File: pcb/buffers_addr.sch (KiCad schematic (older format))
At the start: 24 parts, among them U3 74LVCH162245A, U4 74LVCH162245A

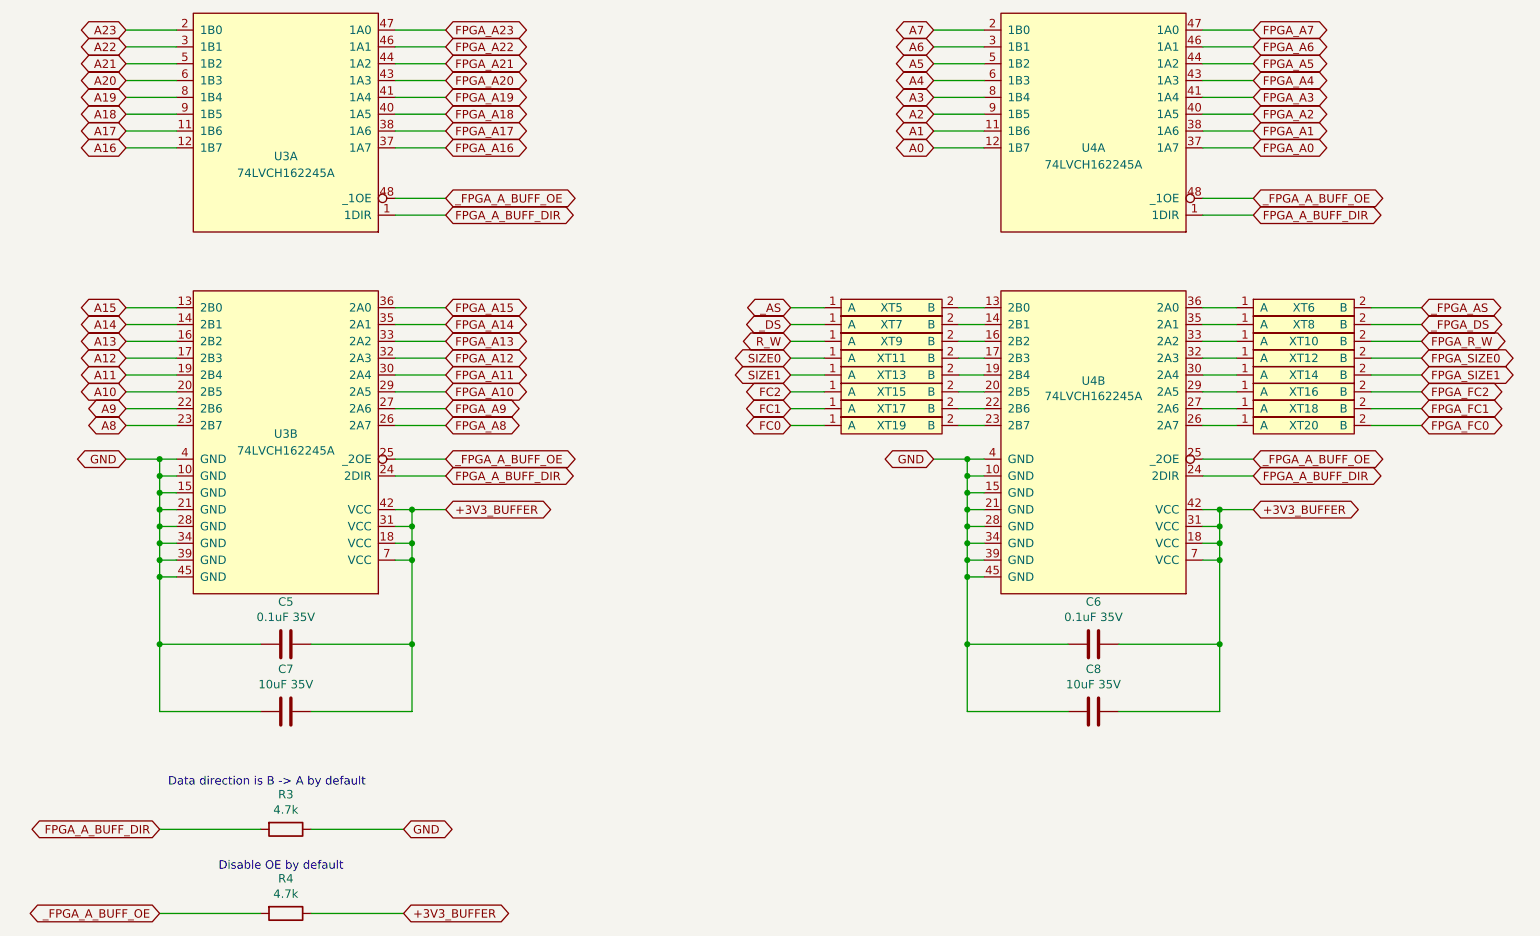
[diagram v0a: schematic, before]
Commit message: working on pcb 2
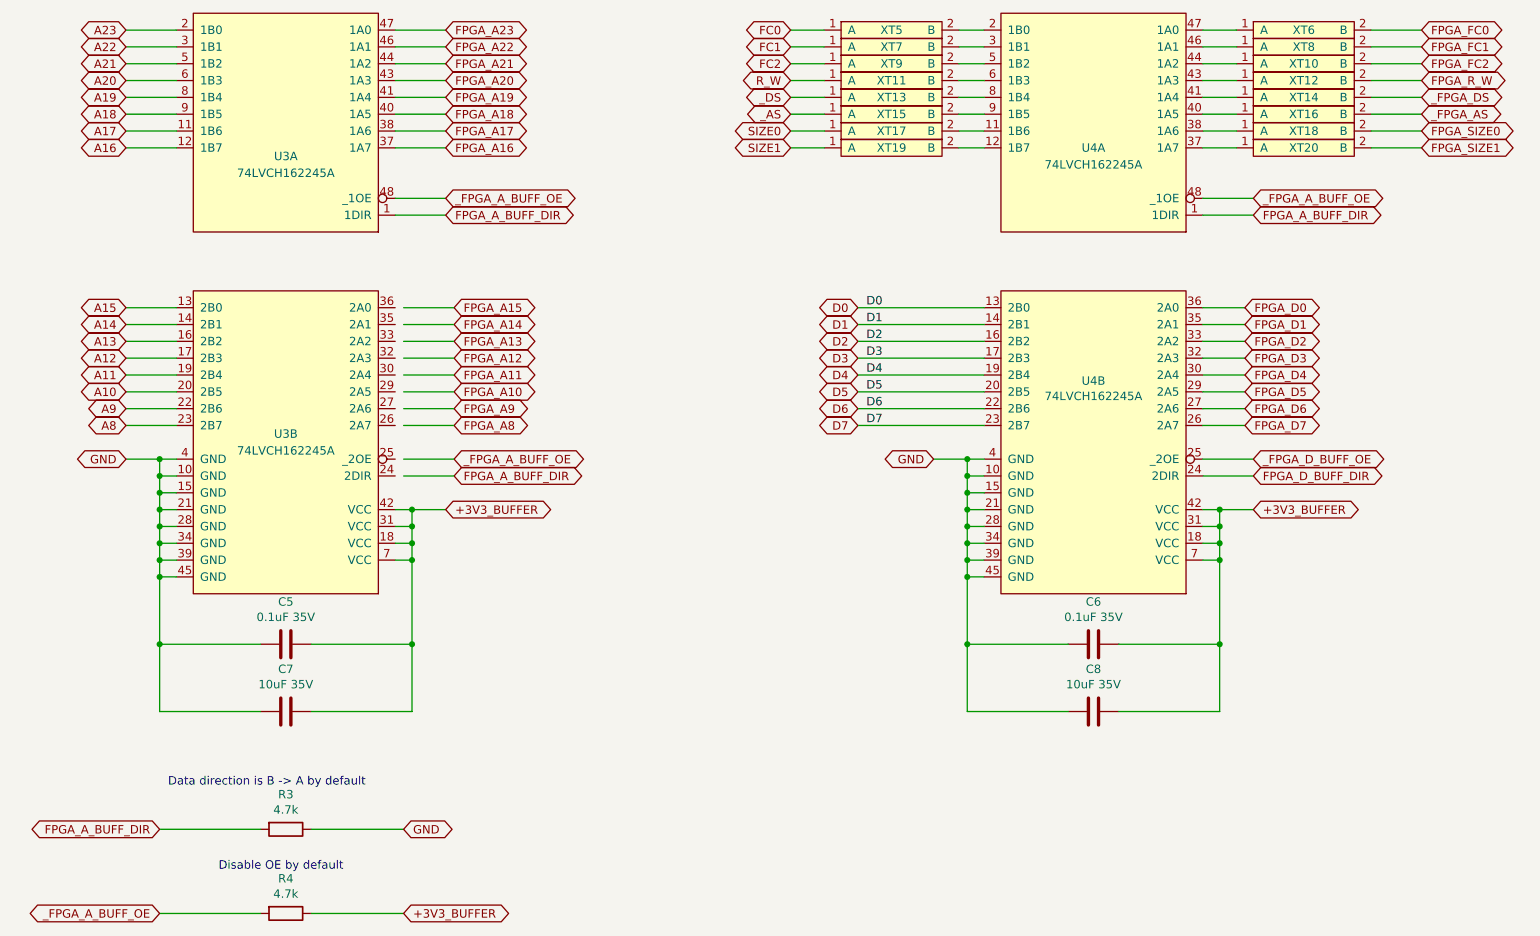
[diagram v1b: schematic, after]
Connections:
- net labels added: D0, D1, D2, D3, D4, D5, D6, D7, FPGA_D0, FPGA_D1, FPGA_D2, FPGA_D3, FPGA_D4, FPGA_D5, FPGA_D6, FPGA_D7, FPGA_D_BUFF_DIR, _FPGA_D_BUFF_OE
- net labels removed: A0, A1, A2, A3, A4, A5, A6, A7, FPGA_A0, FPGA_A1, FPGA_A2, FPGA_A3, FPGA_A4, FPGA_A5, FPGA_A6, FPGA_A7
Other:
- moved on the sheet: XT10, XT11, XT12, XT13, XT14, XT15, XT16, XT17, XT18, XT19, XT20, XT5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

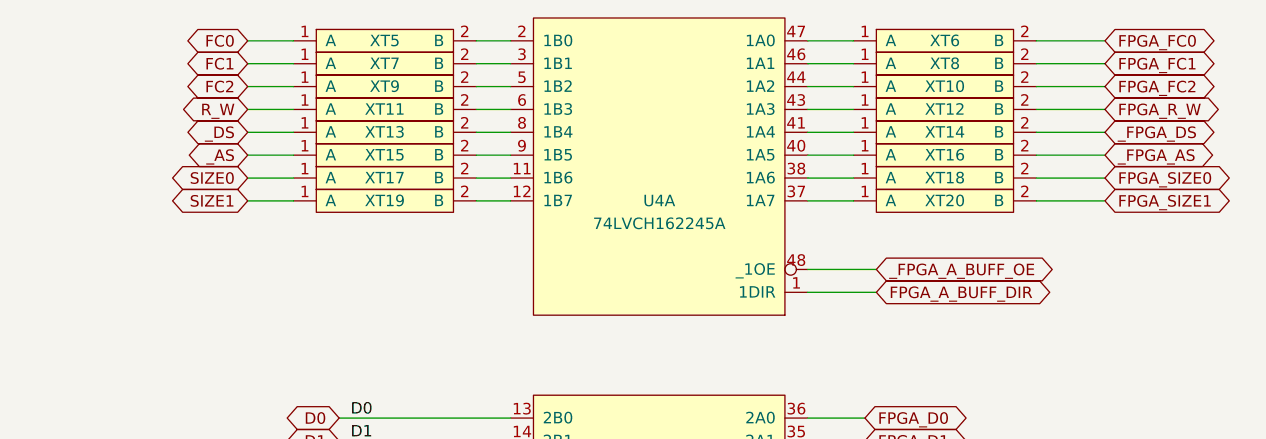
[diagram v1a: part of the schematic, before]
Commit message: working on pcb
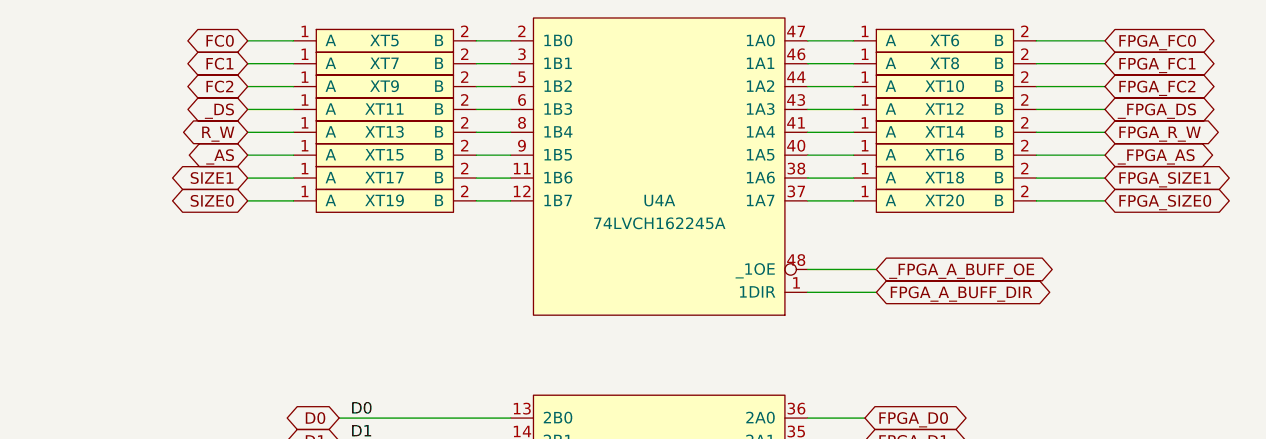
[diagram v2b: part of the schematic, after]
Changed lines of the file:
@@
 	9700 1850 10000 1850
 Wire Wire Line
-	10000 2150 9700 2150
-Wire Wire Line
-	9700 2250 10000 2250
+	10000 2250 9700 2250
+Wire Wire Line
+	9700 2150 10000 2150
 Wire Wire Line
 	10000 1750 9700 1750
@@
 Text GLabel 10000 2050 2    50   BiDi ~ 0
 _FPGA_AS
+Text GLabel 10000 1850 2    50   BiDi ~ 0
+_FPGA_DS
 Text GLabel 10000 1950 2    50   BiDi ~ 0
-_FPGA_DS
-Text GLabel 10000 1850 2    50   BiDi ~ 0
 FPGA_R_W
+Text GLabel 10000 2250 2    50   BiDi ~ 0
+FPGA_SIZE0
 Text GLabel 10000 2150 2    50   BiDi ~ 0
-FPGA_SIZE0
-Text GLabel 10000 2250 2    50   BiDi ~ 0
 FPGA_SIZE1
 Text GLabel 10000 1750 2    50   BiDi ~ 0
@@
 FPGA_FC0
 Wire Wire Line
-	6250 2250 6450 2250
-Wire Wire Line
-	6450 2150 6250 2150
+	6450 2250 6250 2250
 Wire Wire Line
 	6250 1550 6450 1550
@@
 Text GLabel 6250 1750 0    50   BiDi ~ 0
 FC2
-Text GLabel 6250 2250 0    50   BiDi ~ 0
-SIZE1
-Text GLabel 6250 2150 0    50   BiDi ~ 0
-SIZE0
+Text GLabel 6250 1950 0    50   BiDi ~ 0
+R_W
 Text GLabel 6250 1850 0    50   BiDi ~ 0
-R_W
-Text GLabel 6250 1950 0    50   BiDi ~ 0
 _DS
 Text GLabel 6250 2050 0    50   BiDi ~ 0
@@
 Wire Wire Line
 	7400 3900 6650 3900
+Text GLabel 6250 2250 0    50   BiDi ~ 0
+SIZE0
+Text GLabel 6250 2150 0    50   BiDi ~ 0
+SIZE1
+Wire Wire Line
+	6250 2150 6450 2150
 $EndSCHEMATC

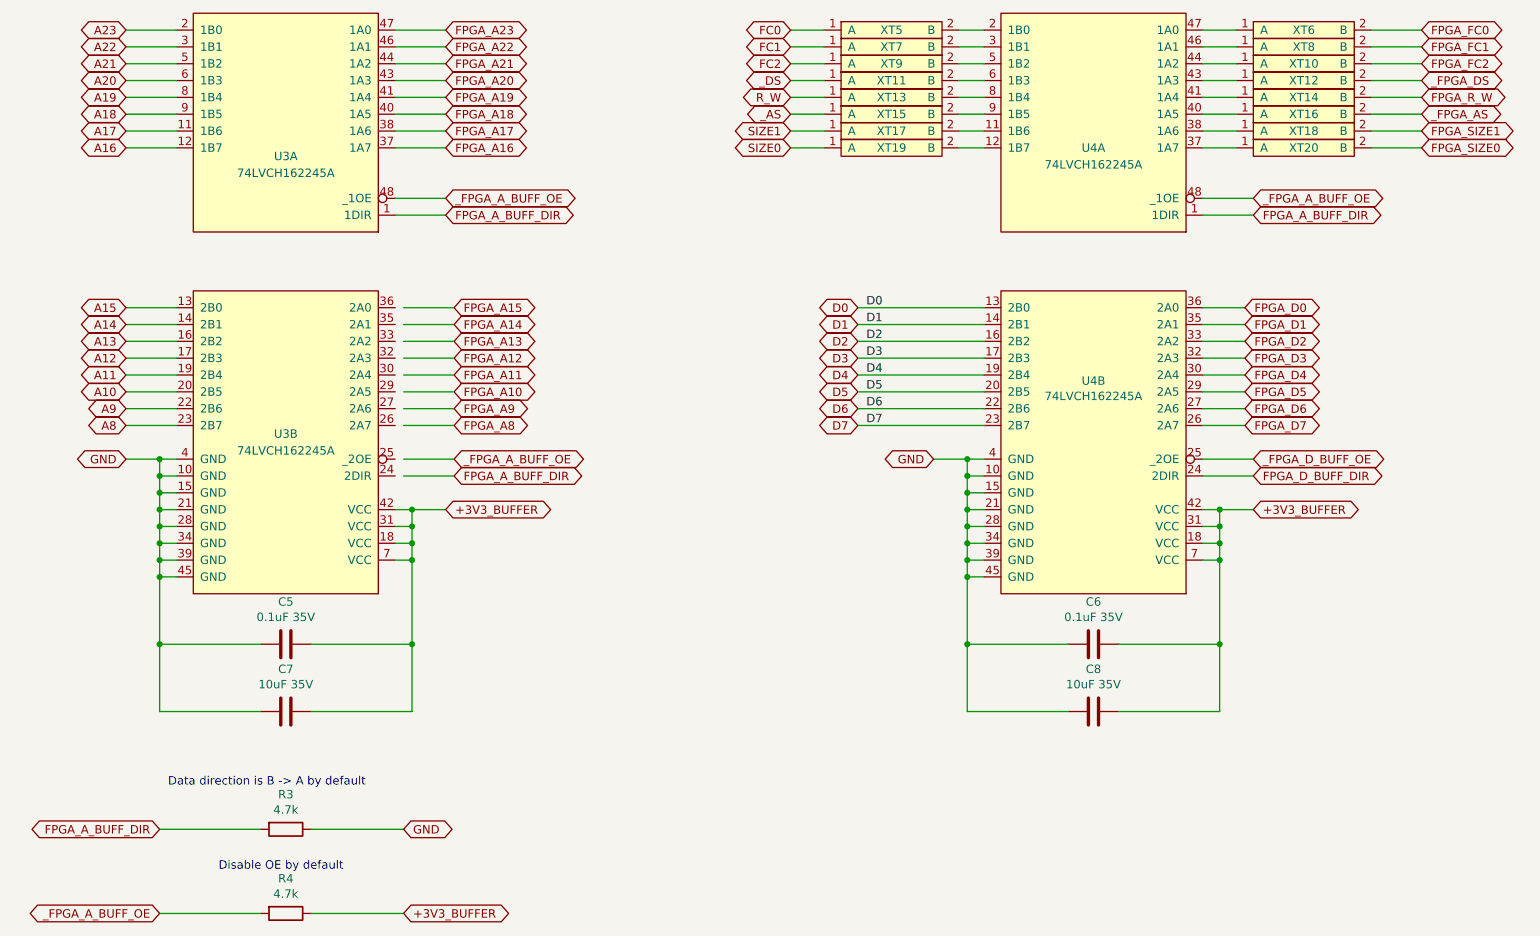
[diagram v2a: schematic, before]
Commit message: Board pcb updated
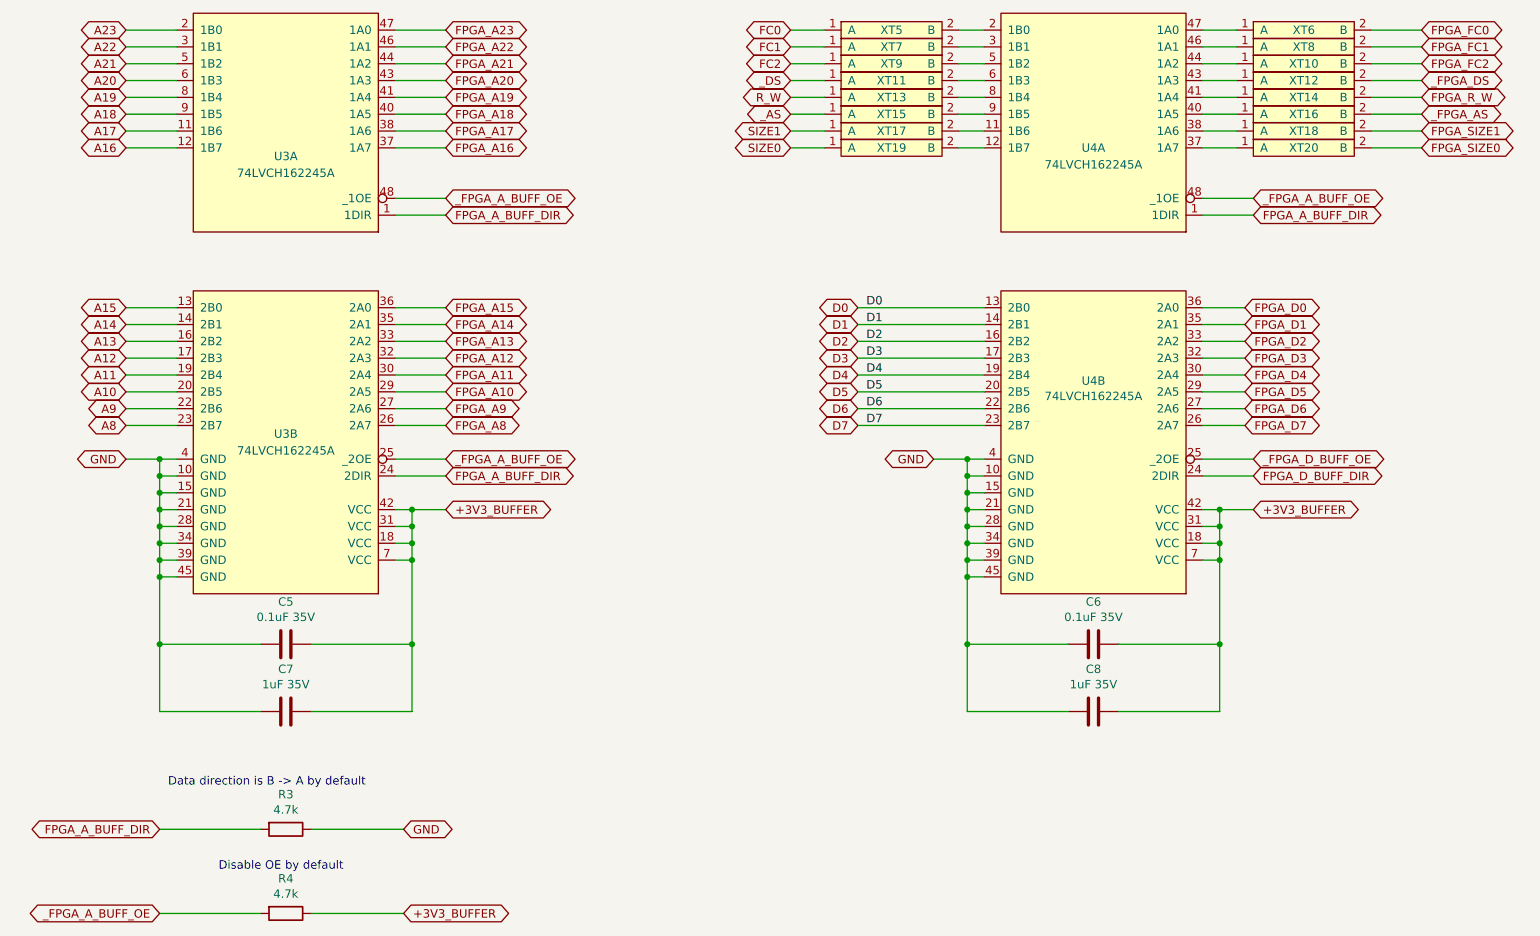
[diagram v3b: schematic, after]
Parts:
- C7, C8: value 10uF 35V -> 1uF 35V; footprint Capacitor_SMD:C_1210_3225Metric_Pad1.42x2.65mm_HandSolder -> Capacitor_SMD:C_0805_2012Metric_Pad1.15x1.40mm_HandSolder
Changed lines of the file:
@@
 	2300 3900 2600 3900
 Wire Wire Line
-	3950 3800 4250 3800
-Wire Wire Line
-	4250 3900 3950 3900
-Wire Wire Line
-	3950 3600 4250 3600
-Wire Wire Line
-	4250 4100 3950 4100
-Wire Wire Line
-	3950 4200 4250 4200
-Wire Wire Line
-	4250 3700 3950 3700
+	3900 3800 4200 3800
+Wire Wire Line
+	4200 3900 3900 3900
+Wire Wire Line
+	3900 3600 4200 3600
+Wire Wire Line
+	4200 4100 3900 4100
+Wire Wire Line
+	3900 4200 4200 4200
+Wire Wire Line
+	4200 3700 3900 3700
 Wire Wire Line
 	3900 1550 4200 1550
@@
 	4200 2650 3900 2650
 Wire Wire Line
-	3950 3200 4250 3200
-Wire Wire Line
-	4250 3300 3950 3300
-Wire Wire Line
-	3950 3400 4250 3400
-Wire Wire Line
-	4250 3500 3950 3500
+	3900 3200 4200 3200
+Wire Wire Line
+	4200 3300 3900 3300
+Wire Wire Line
+	3900 3400 4200 3400
+Wire Wire Line
+	4200 3500 3900 3500
 Wire Wire Line
 	7400 4100 7300 4100
@@
 P 3250 5600
 F 0 "C7" V 3502 5600 50  0000 C CNN
-F 1 "10uF 35V" V 3411 5600 50  0000 C CNN
-F 2 "Capacitor_SMD:C_1210_3225Metric_Pad1.42x2.65mm_HandSolder" H 3288 5450 50  0001 C CNN
+F 1 "1uF 35V" V 3411 5600 50  0000 C CNN
+F 2 "Capacitor_SMD:C_0805_2012Metric_Pad1.15x1.40mm_HandSolder" H 3288 5450 50  0001 C CNN
 F 3 "~" H 3250 5600 50  0001 C CNN
 	1    3250 5600
@@
 P 8050 5600
 F 0 "C8" V 8302 5600 50  0000 C CNN
-F 1 "10uF 35V" V 8211 5600 50  0000 C CNN
-F 2 "Capacitor_SMD:C_1210_3225Metric_Pad1.42x2.65mm_HandSolder" H 8088 5450 50  0001 C CNN
+F 1 "1uF 35V" V 8211 5600 50  0000 C CNN
+F 2 "Capacitor_SMD:C_0805_2012Metric_Pad1.15x1.40mm_HandSolder" H 8088 5450 50  0001 C CNN
 F 3 "~" H 8050 5600 50  0001 C CNN
 	1    8050 5600
@@
 Text GLabel 4200 2550 2    50   BiDi ~ 0
 _FPGA_A_BUFF_OE
-Text GLabel 4250 4100 2    50   BiDi ~ 0
+Text GLabel 4200 4100 2    50   BiDi ~ 0
 _FPGA_A_BUFF_OE
 Text GLabel 9000 4100 2    50   BiDi ~ 0
@@
 Text GLabel 2500 6800 0    50   BiDi ~ 0
 _FPGA_A_BUFF_OE
-Text GLabel 4250 4200 2    50   BiDi ~ 0
+Text GLabel 4200 4200 2    50   BiDi ~ 0
 FPGA_A_BUFF_DIR
 Text GLabel 9000 2650 2    50   BiDi ~ 0
@@
 Text GLabel 4200 2250 2    50   BiDi ~ 0
 FPGA_A16
-Text GLabel 4250 3200 2    50   BiDi ~ 0
+Text GLabel 4200 3200 2    50   BiDi ~ 0
 FPGA_A15
-Text GLabel 4250 3300 2    50   BiDi ~ 0
+Text GLabel 4200 3300 2    50   BiDi ~ 0
 FPGA_A14
-Text GLabel 4250 3400 2    50   BiDi ~ 0
+Text GLabel 4200 3400 2    50   BiDi ~ 0
 FPGA_A13
-Text GLabel 4250 3500 2    50   BiDi ~ 0
+Text GLabel 4200 3500 2    50   BiDi ~ 0
 FPGA_A12
-Text GLabel 4250 3600 2    50   BiDi ~ 0
+Text GLabel 4200 3600 2    50   BiDi ~ 0
 FPGA_A11
-Text GLabel 4250 3700 2    50   BiDi ~ 0
+Text GLabel 4200 3700 2    50   BiDi ~ 0
 FPGA_A10
-Text GLabel 4250 3800 2    50   BiDi ~ 0
+Text GLabel 4200 3800 2    50   BiDi ~ 0
 FPGA_A9
-Text GLabel 4250 3900 2    50   BiDi ~ 0
+Text GLabel 4200 3900 2    50   BiDi ~ 0
 FPGA_A8
 Text GLabel 10000 2050 2    50   BiDi ~ 0
